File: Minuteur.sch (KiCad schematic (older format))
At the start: 44 parts, among them J1 Screw_Terminal_01x02, J2 ICSP, J4 Conn_01x10, J5 output, J6 Screw_Terminal_01x03, Q1 BC818, SW1 Rotary_Encoder_Switch, SW2 SW_Push_SPDT_2Leds, U1 ATmega328P-AU, U2 LD1117S50TR_SOT223, U3 MAX7219, U4 LTV-817S, U5 CC56-12EWA, U6 Piezo_sounder, Y1 16MHz

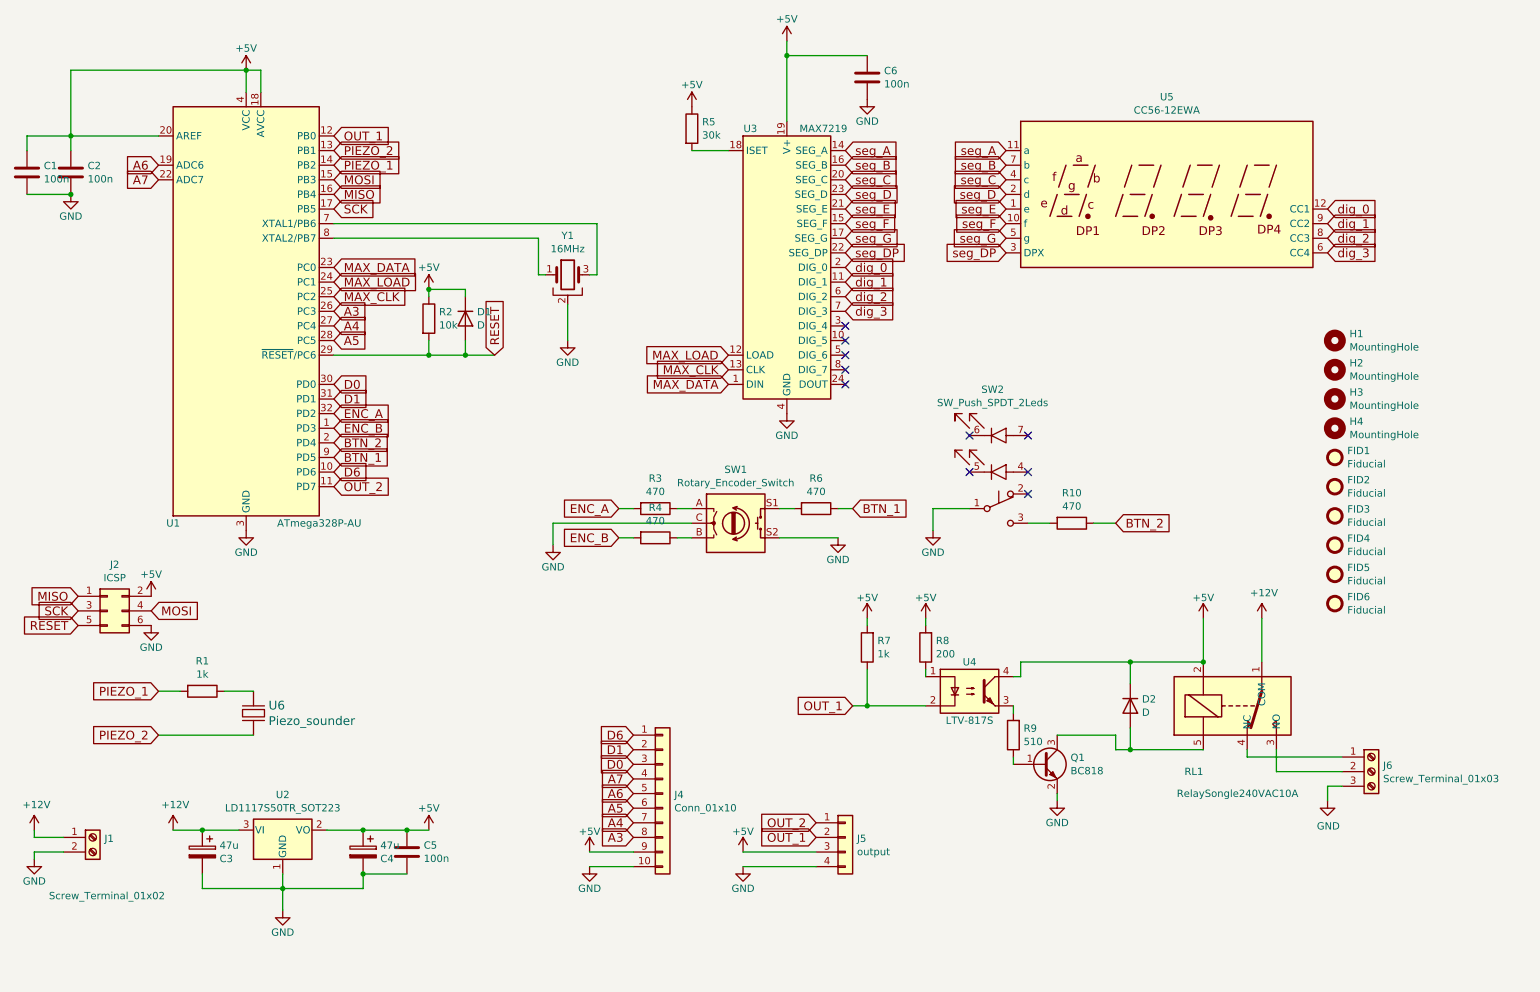
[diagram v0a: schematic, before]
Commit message: AC version ready for fab.
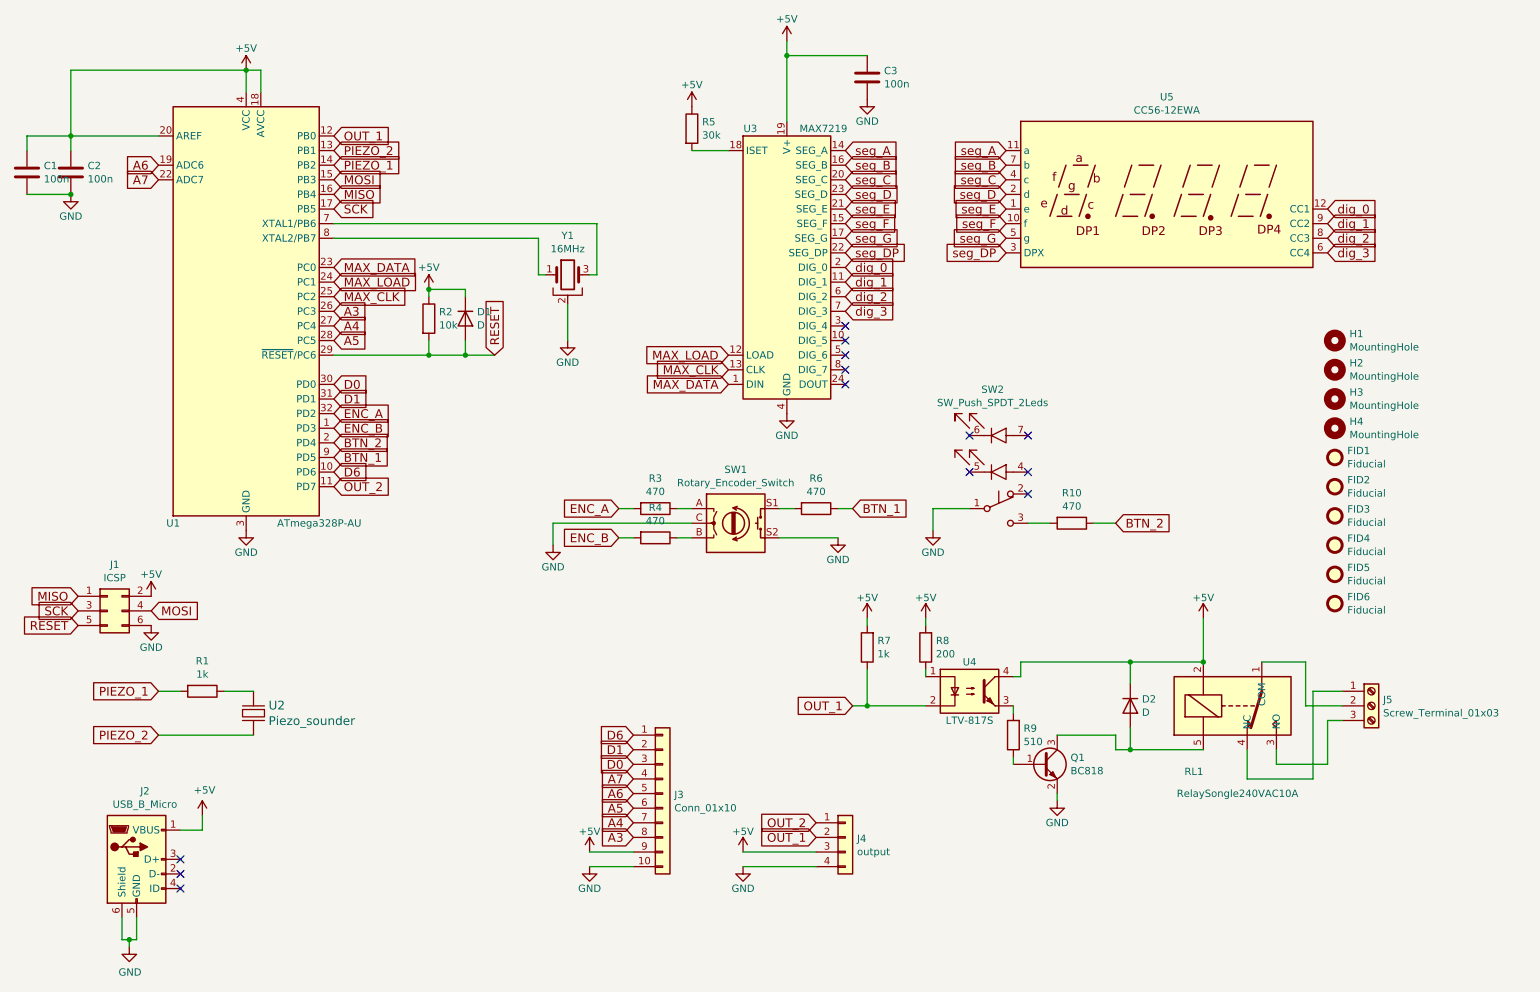
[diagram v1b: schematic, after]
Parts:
- removed C3, C4: 47u, Capacitor_SMD:CP_Elec_6.3x5.3, symbol Device:CP
- removed C5: 100n, Capacitor_SMD:C_0805_2012Metric, symbol Device:C
- removed J1: Screw_Terminal_01x02, Connector_Phoenix_MSTB:PhoenixContact_MSTBVA_2,5_2-G-5,08_1x02_P5.08mm_Vertical, symbol Connector:Screw_Terminal_01x02
- removed U2: LD1117S50TR_SOT223, Package_TO_SOT_SMD:SOT-223-3_TabPin2, symbol Regulator_Linear:LD1117S50TR_SOT223
- added J2: USB_B_Micro, Connector_USB:USB_Micro-B_Amphenol_10118194_Horizontal, symbol Connector:USB_B_Micro
- renumbered C6 to C3, J2 to J1, J4 to J3, J5 to J4, J6 to J5, U6 to U2
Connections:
- net +12V is gone; now on an unnamed net: RL1.1 (COM)
- net +5V: now also J2.1 (VBUS)
- net GND: now also J2.5 (GND), J2.6 (Shield); no longer J5.3 (Pin_3)
- net at J5.2 (Pin_2): no longer RL1.3 (NO)
- new net: J5.3 (Pin_3), RL1.3 (NO)
- no-connect marks 10 -> 13
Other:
- moved on the sheet: J5
